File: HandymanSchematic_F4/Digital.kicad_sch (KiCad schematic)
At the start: 45 parts, among them J1 SWD Header, J2 Footswitch, J3 TunerIn, J4 TuneThru, J5 GateIn, J6 GateOut, J7 PowerJack, Q2 2N7002, Q3 2N7002, SW1 RST, SW2 BYP, U1 SH1106, U3 STM32F411RETx, U4 AMS1117, Y1 16MHz

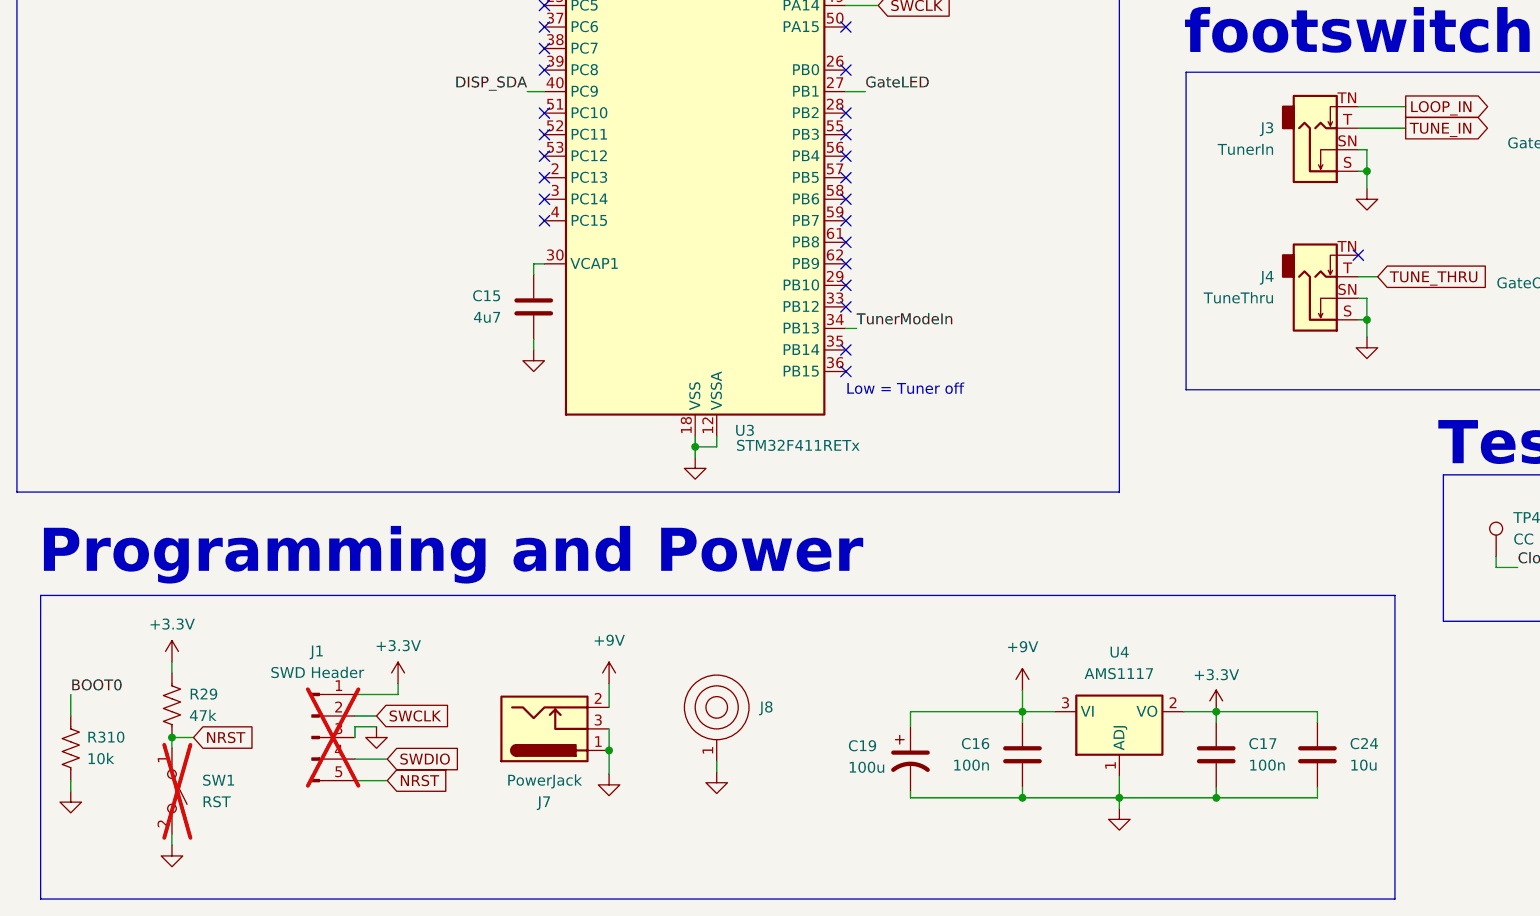
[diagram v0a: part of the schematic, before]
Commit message: noise schematic tweaks
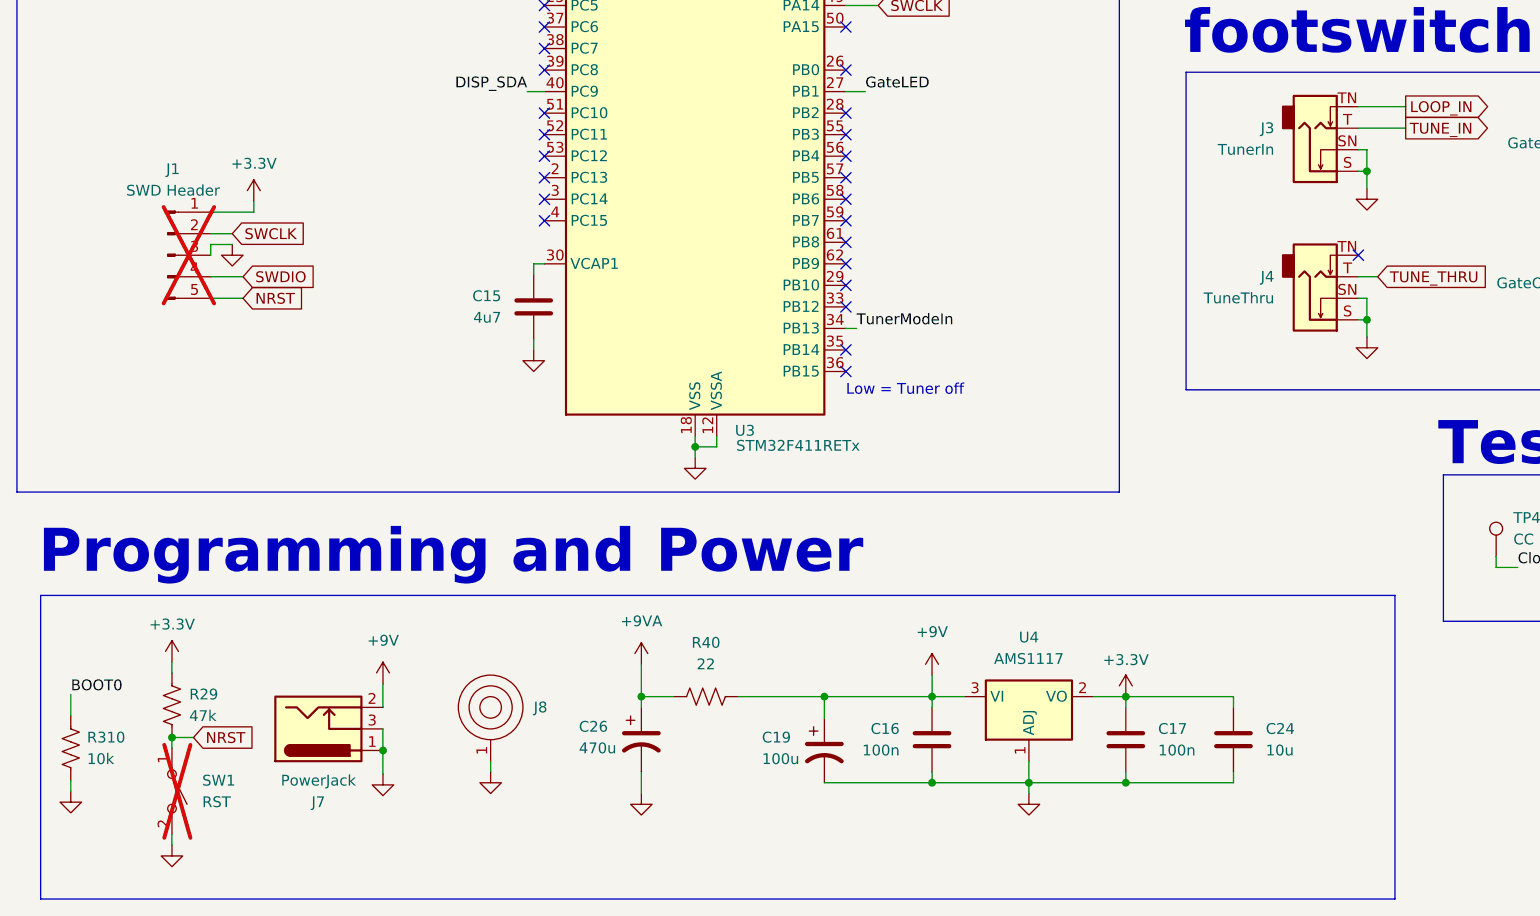
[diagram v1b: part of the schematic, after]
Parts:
- added C26: 470u, Capacitor_THT:CP_Radial_D6.3mm_P2.50mm, symbol Device:C_Polarized_US
- added R40: 22, Resistor_SMD:R_0805_2012Metric, symbol Device:R_US
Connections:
- net +9V: now also R40.2
- net GND: now also C26.2
- new net +9VA: C26.1, R40.1
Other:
- moved on the sheet: C16, C17, C19, C24, J1, J7, J8, U4
